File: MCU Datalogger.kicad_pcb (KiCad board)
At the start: 2 copper layers, 50 x 30 mm, 29 parts, among them J1 Conn_01x04_Pin, J2 Conn_01x04_Pin, J3 Conn_01x09_Pin, J4 Conn_02x03_Odd_Even, U1 DS1337S_, U2 ATMEGA328P-AU, U3 24LC1025, U4 24LC1025, Y1 32.768 KHz, Y2 16MHz

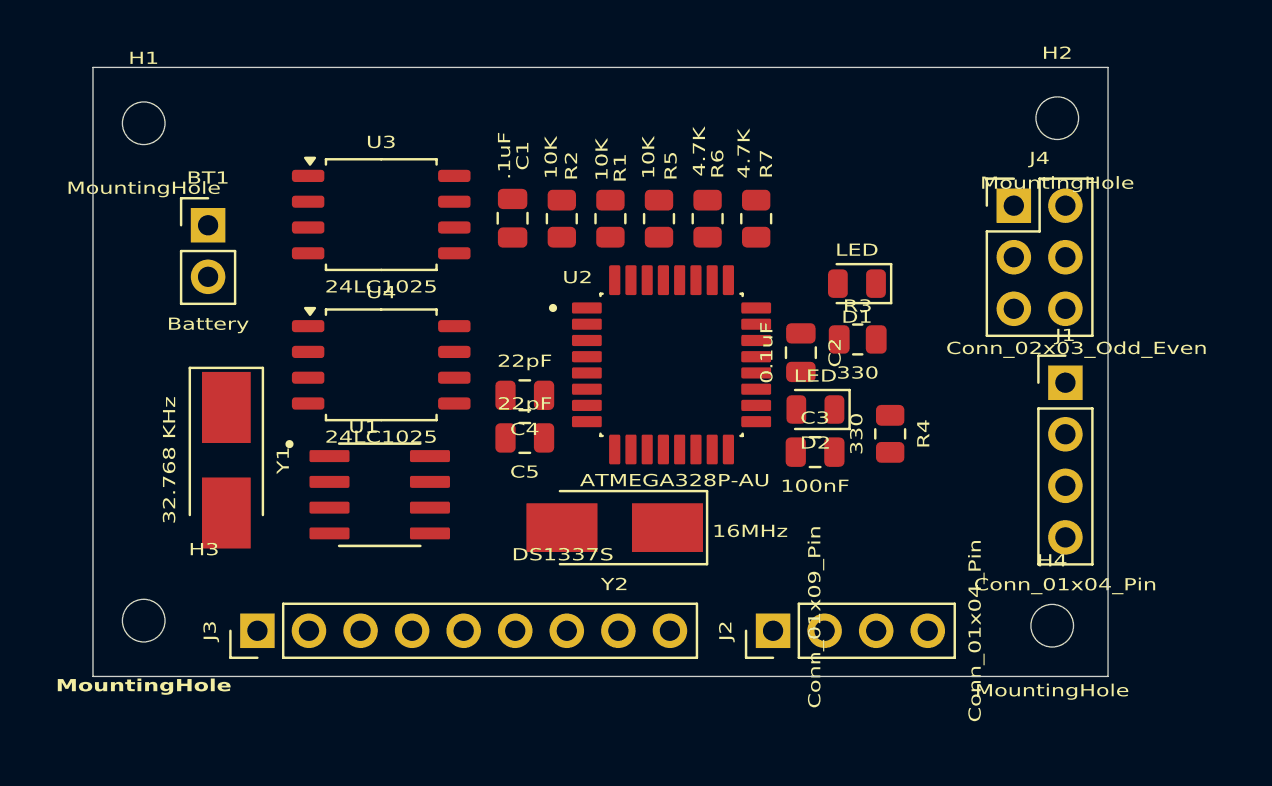
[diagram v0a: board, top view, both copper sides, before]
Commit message: Initial Routing
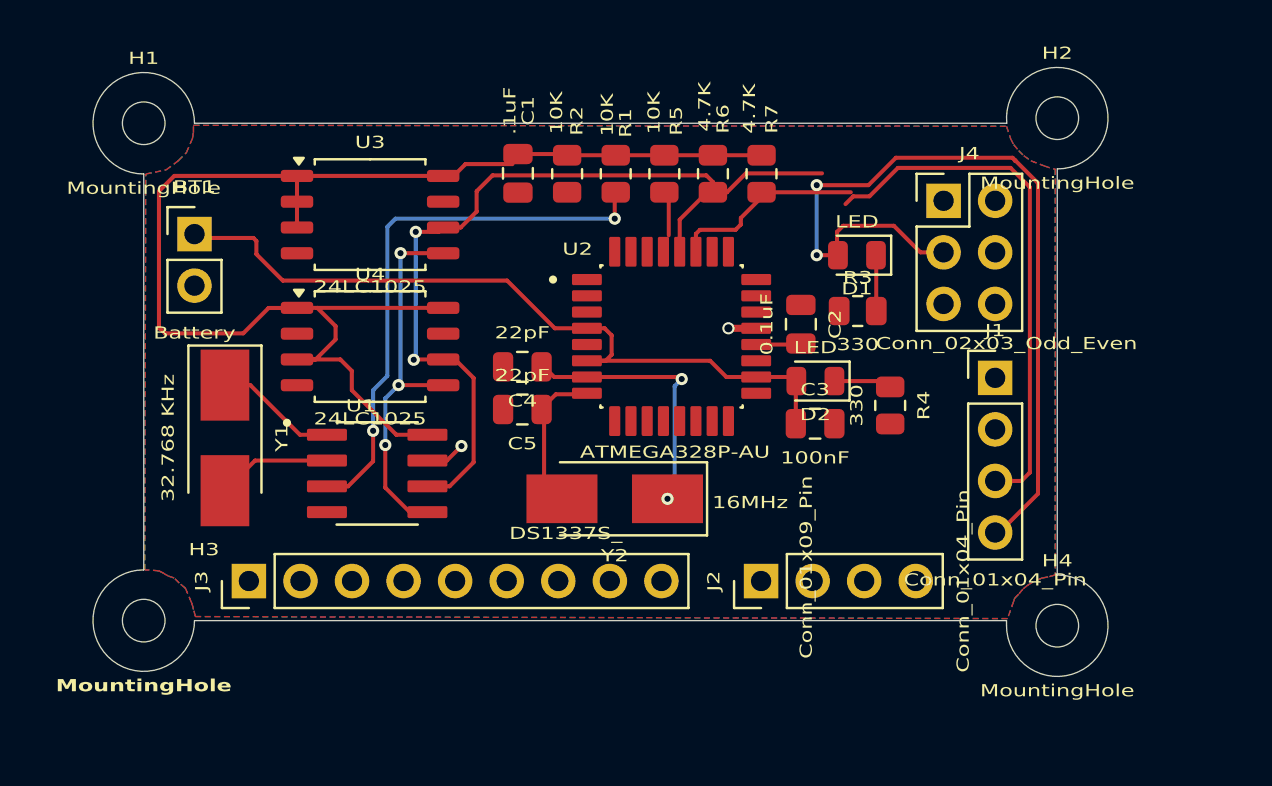
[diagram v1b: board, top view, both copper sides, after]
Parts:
- moved J1 3.47 mm to (131.9, 72.5)
- moved J4 3.47 mm to (129.4, 63.8)
- moved J2 2.52 mm to (120.4, 82.5)
- moved J3 2.49 mm to (95.2, 82.5)
- moved C1 2.23 mm to (108.4, 62.5)
- moved R1 2.23 mm to (113.2, 62.5)
- moved R2 2.23 mm to (110.9, 62.5)
- moved R5 2.23 mm to (115.6, 62.5)
- moved R6 2.23 mm to (118.0, 62.5)
- moved R7 2.23 mm to (120.4, 62.5)
- moved Y2 1.42 mm to (113.2, 78.5)
- moved C4 1.41 mm to (108.7, 72.0)
- moved C5 1.41 mm to (108.7, 74.1)
- moved C3 1.40 mm to (123.1, 74.8)
- moved D1 1.40 mm to (125.1, 66.5)
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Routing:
- net /SCK: track 0.00 -> 85.0 mm, vias 0 -> 4
- net /VCC: track 0.00 -> 67.0 mm
- net /SDA: track 0.00 -> 54.6 mm, vias 0 -> 3
- net Net-(BT1-+): track 0.00 -> 38.1 mm
- net Net-(U1-~{INTA}): track 0.00 -> 27.3 mm, vias 0 -> 2
- net Net-(U2-PB6): track 0.00 -> 13.2 mm, vias 0 -> 2
- net Net-(U2-PB7): track 0.00 -> 7.06 mm
- net Net-(U1-X1): track 0.00 -> 6.04 mm
- net Net-(U1-X2): track 0.00 -> 5.64 mm
- net Net-(D2-K): track 0.00 -> 2.87 mm
- net Net-(D1-K): track 0.00 -> 2.76 mm
- net Net-(U2-AREF): track 0.00 -> 2.22 mm
- net /RESET: track 0.00 -> 2.21 mm
- net Net-(U1-SQW/~INT): track 0.00 -> 1.97 mm, vias 0 -> 1
- net GND: track 0.00 -> 1.37 mm, vias 0 -> 1
- added copper zone on B.Cu, net GND
- added copper zone on F.Cu, net GND
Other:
- outline, holes or cut-outs redrawn
